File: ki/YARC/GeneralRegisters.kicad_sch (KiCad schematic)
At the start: 13 parts, among them U71 74LS670, U72 74LS670, U73 74LS157, U74 74LS670, U75 74LS670, U76 74LS157, U77 74LS670, U78 74LS670, U79 74LS157, U80 74LS670, U81 74LS670, U82 74LS157, U96 74LS32

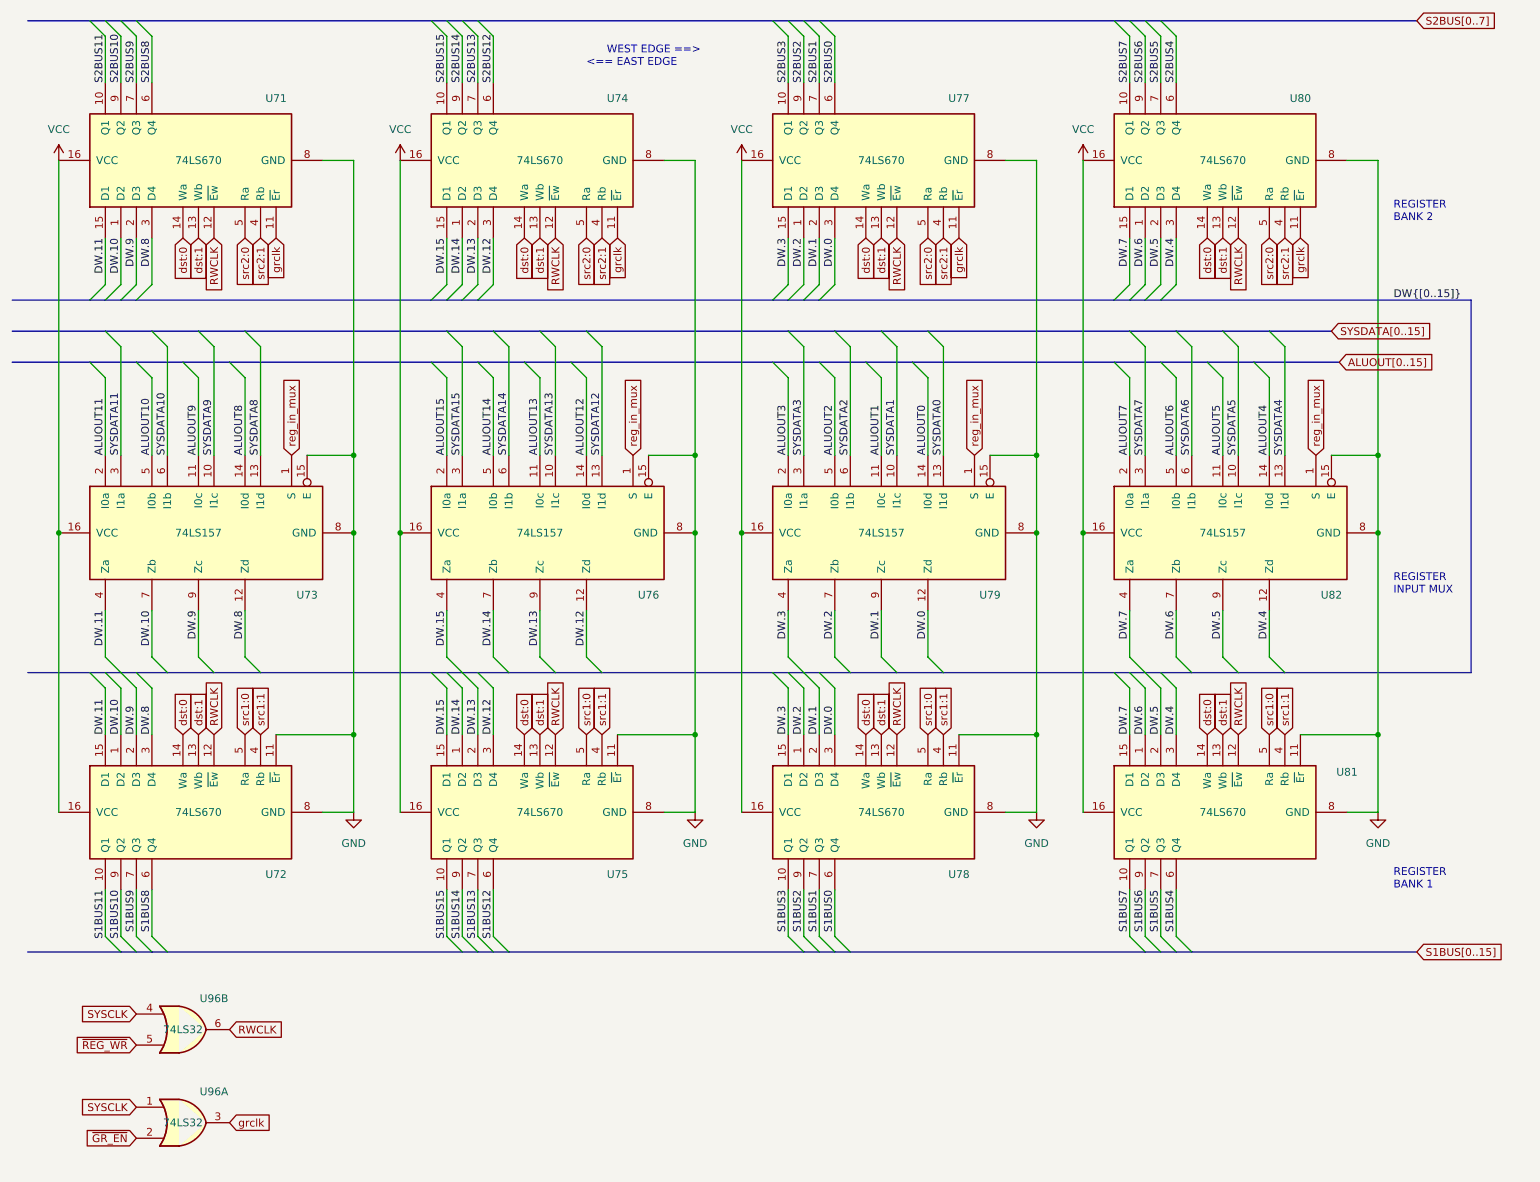
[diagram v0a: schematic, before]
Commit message: Continuing cleanup of schematic
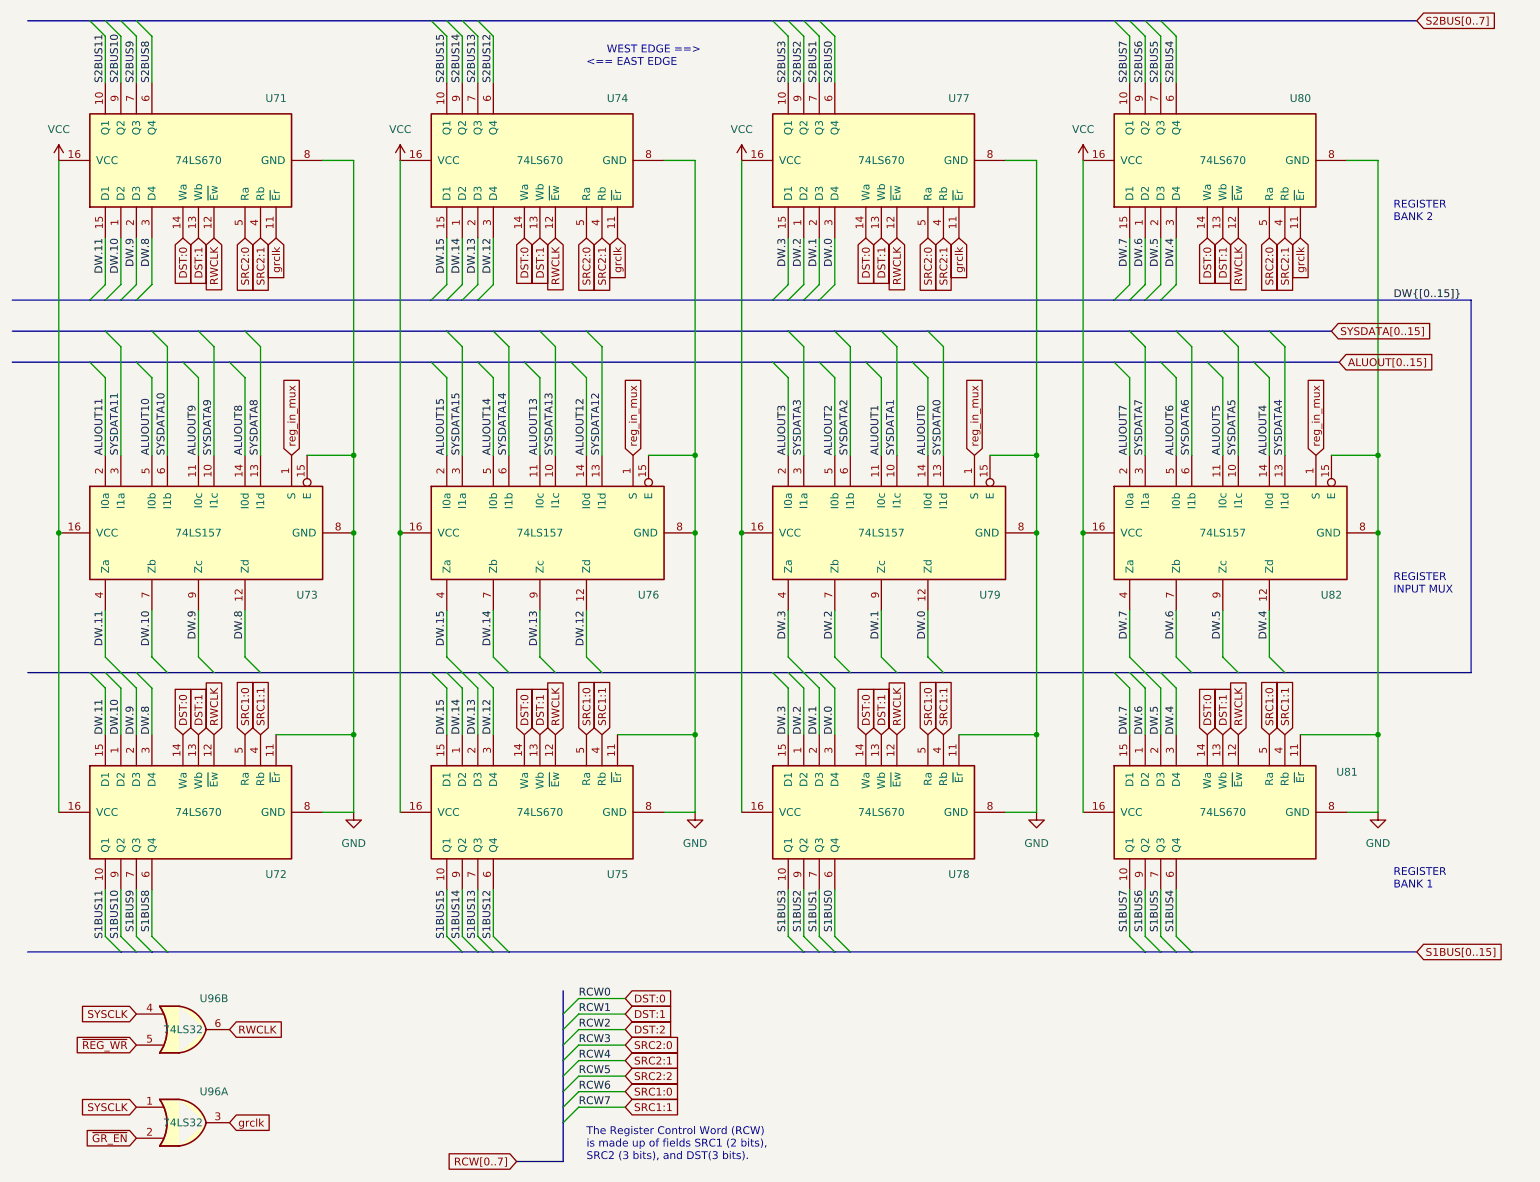
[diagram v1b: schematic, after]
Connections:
- net dst:0 renamed DST:0
- net dst:1 renamed DST:1
- net src1:0 renamed SRC1:0
- net src1:1 renamed SRC1:1
- net src2:0 renamed SRC2:0
- net src2:1 renamed SRC2:1
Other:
- note added: "The Register Control Word (RCW) is made up of fields SRC1 (2 bits), SRC2 (3 bits), and DST(3 bits)."
